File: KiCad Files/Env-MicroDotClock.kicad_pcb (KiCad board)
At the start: 2 copper layers, 90 x 65.2 mm, 39 parts, among them IC1 IS31FL3730-QFLS2-TR, IC2 IS31FL3730-QFLS2-TR, IC3 IS31FL3730-QFLS2-TR, IC4 IS31FL3730-QFLS2-TR, M1 LTP-305G, M2 LTP-305G, M3 LTP-305G, M4 LTP-305G, M5 LTP-305G, M6 LTP-305G, M7 LTP-305G, M8 LTP-305G, Q1 2SC1815, SW1 SW_Push, SW2 SW_Push, SW3 SW_Push, SW4 SW_Push, U1 Pico, U3 DS3231M

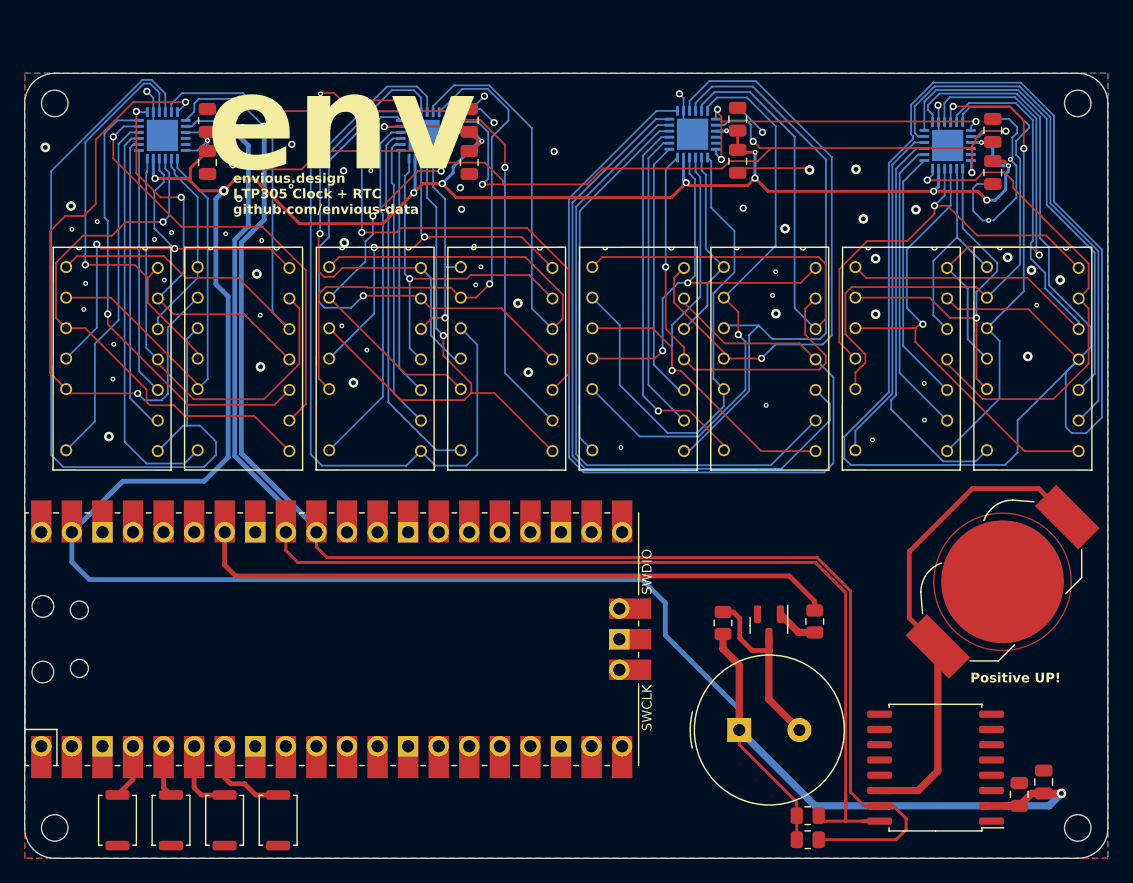
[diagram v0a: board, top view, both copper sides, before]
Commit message: some fixes and adjustments.
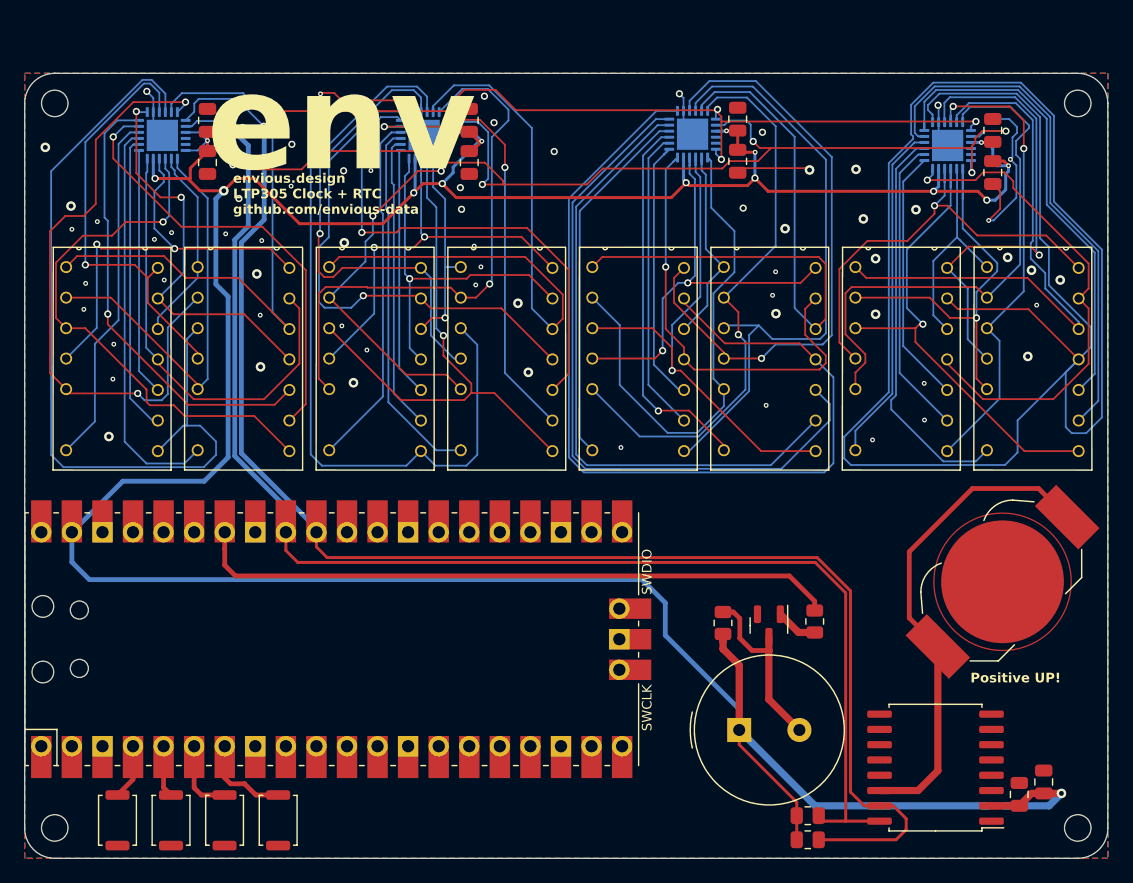
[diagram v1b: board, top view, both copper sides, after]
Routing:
- net I2C_SDA: track 169.2 -> 193.9 mm
- net GND: track 55.6 -> 46.8 mm
- net IC4R1: track 31.3 -> 33.8 mm
- net I2C_SCL: track 208.1 -> 205.9 mm
- net Buzzer GPIO: track 53.8 -> 55.5 mm
- net IC4R3: track 39.2 -> 40.7 mm
- net IC2R4: track 33.6 -> 35.1 mm
- net GPIO5: track 7.66 -> 8.98 mm
- net IC4R4: track 36.0 -> 37.1 mm
- net +5V: track 282.3 -> 283.3 mm
- net IC4C6: track 38.7 -> 39.5 mm
- net IC3R4: track 35.1 -> 35.7 mm
- net IC2C3: track 64.8 -> 65.5 mm
- net IC3R6: track 21.8 -> 22.4 mm
- net IC2C4: track 39.7 -> 40.3 mm
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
